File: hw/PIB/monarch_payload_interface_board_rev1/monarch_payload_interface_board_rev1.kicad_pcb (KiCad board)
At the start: 4 copper layers, 96 x 89.9 mm, 187 parts, among them J1 5037630291, J10 5037630491, J11 5037630691, J12 5037630691, J13 5037630491, J14 5037630491, J15 5037630691, J16 20021121-00008C4LF, J2 5037630291, J3 5037630691, J4 5037630691, J5 5037630691, J6 5037630691, J7 5037630691, J8 5037630691, J9 5037630491, Q1 FZT600TA, Q10 FZT600TA, Q11 FZT600TA, Q12 FZT600TA, Q13 FZT600TA, Q14 FZT600TA, Q15 FZT600TA, Q16 FZT600TA, Q17 FZT600TA, Q18 FZT600TA, Q19 FZT600TA, Q2 FZT600TA, Q3 FZT600TA, Q4 FZT600TA, Q5 FZT600TA, Q6 FZT600TA, Q7 FZT600TA, Q8 FZT600TA, Q9 FZT600TA, U1 Payload, U10 AD7124-8BCPZ-RL, U11 WSK06121L000FEA, U12 WSK06121L000FEA, U13 WSK06121L000FEA, U14 WSK06121L000FEA, U2 STM32L4A6VGTx, U3 MAX31856MUD_T, U4 TPS61088QRHLRQ1, U5 MAX31856MUD_T, U6 MAX31856MUD_T, U7 MAX31856MUD_T, U8 MAX31856MUD_T, U9 AD7124-8BCPZ-RL

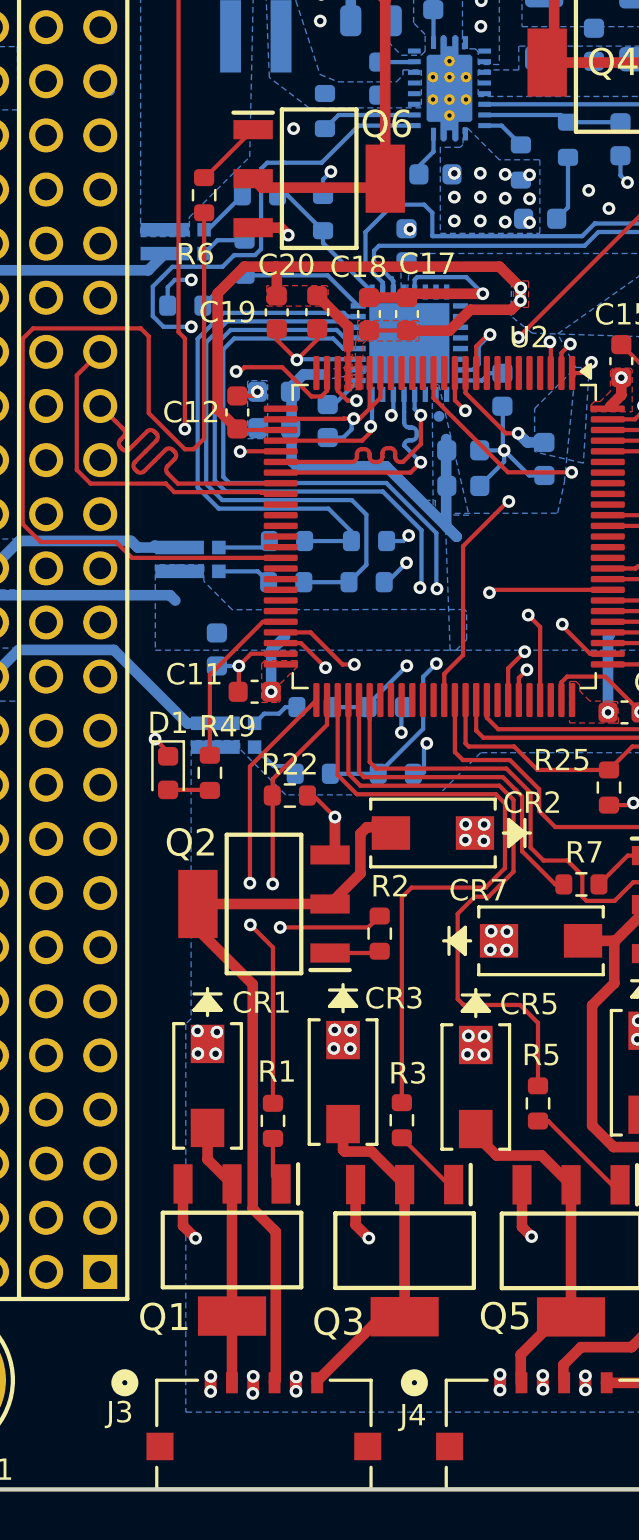
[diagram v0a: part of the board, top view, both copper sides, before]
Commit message: more minor tweaks
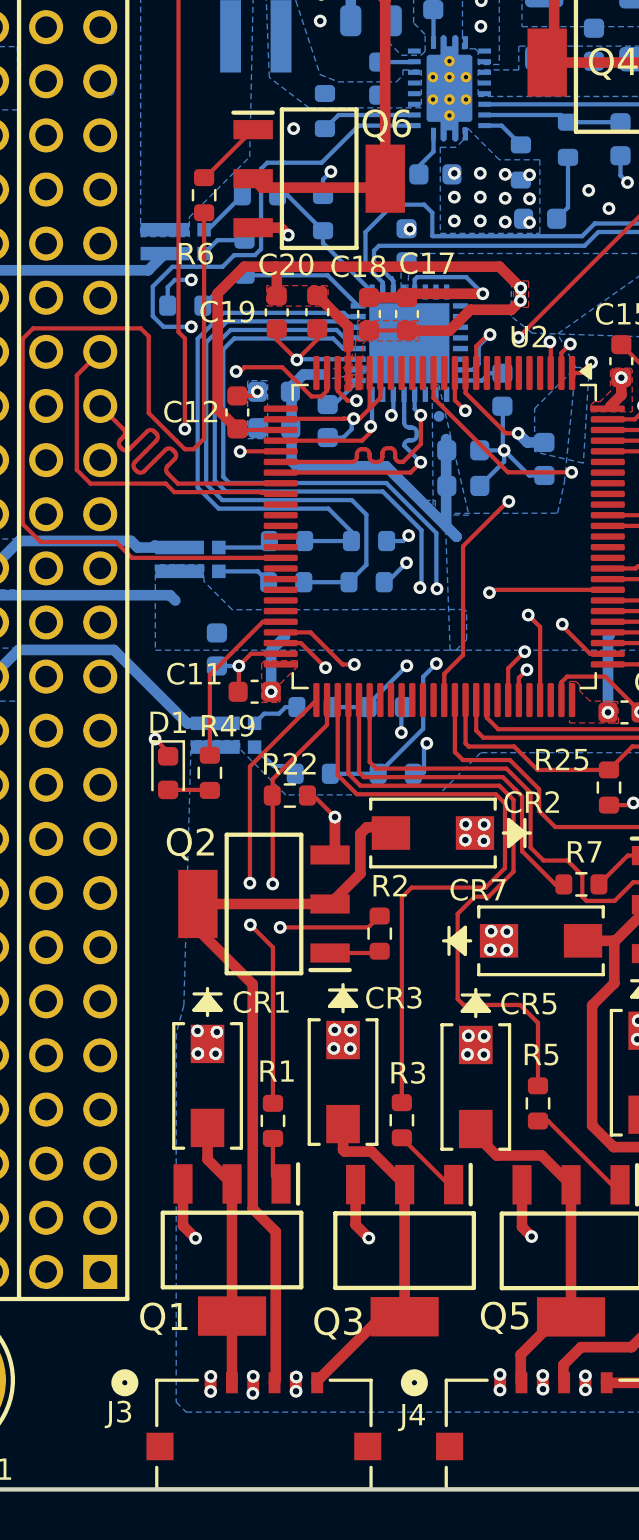
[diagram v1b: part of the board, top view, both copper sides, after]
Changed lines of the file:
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@@
 		(polygon
 			(pts
-				(xy 51.29 70.12) (xy 51.29 83.17) (xy 51.04 83.42) (xy 51.04 101.62) (xy 51.06 101.64) (xy 121.15 101.64)
+				(xy 51.29 70.12) (xy 50.95 82.55) (xy 50.59 83.87) (xy 50.59 101.17) (xy 51.06 101.64) (xy 121.15 101.64)
 				(xy 121.51 101.28) (xy 121.51 70.69) (xy 64.88 70.69) (xy 62.9 72.67) (xy 55.73 72.67) (xy 53.57 70.51)
 				(xy 53.57 70.12)
@@
 			(pts
 				(xy 62.9832 46.3172) (xy 67.6314 46.3172) (xy 67.6568 46.2918) (xy 67.6568 42.8882) (xy 67.6314 42.8628)
-				(xy 65.7518 42.8628) (xy 64.2532 41.3642) (xy 64.05 41.3642) (xy 64.05 42.1516) (xy 63.923 42.2786)
+				(xy 65.7518 42.8628) (xy 64.2532 41.3642) (xy 64.05 41.3642) (xy 64.05 41.9516) (xy 63.723 42.2786)
 				(xy 62.9832 42.2786)
 			)
